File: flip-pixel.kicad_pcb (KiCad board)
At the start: 2 copper layers, 152.4 x 127 mm, 179 parts, among them J1 Barrel-Jack, Q1 DMN62D0U-7, Q10 STS8DN6LF6AG, Q11 DMN62D0U-7, Q12 DMN62D0U-7, Q13 STS8DN6LF6AG, Q14 DMN62D0U-7, Q15 DMN62D0U-7, Q16 STS8DN6LF6AG, Q17 DMN62D0U-7, Q18 DMN62D0U-7, Q19 STS8DN6LF6AG, Q2 DMN62D0U-7, Q20 DMN62D0U-7, Q21 DMN62D0U-7, Q22 STS8DN6LF6AG, Q23 DMN62D0U-7, Q24 DMN62D0U-7, Q25 STS8DN6LF6AG, Q26 DMN62D0U-7, Q27 DMN62D0U-7, Q28 STS8DN6LF6AG, Q29 DMN62D0U-7, Q3 DMN62D0U-7, Q30 DMN62D0U-7, Q31 STS8DN6LF6AG, Q4 STS8DN6LF6AG, Q5 DMN62D0U-7, Q6 DMN62D0U-7, Q7 STS8DN6LF6AG, Q8 DMN62D0U-7, Q9 DMN62D0U-7, U1 LM2665M6, U2 ESP32_DevBoard

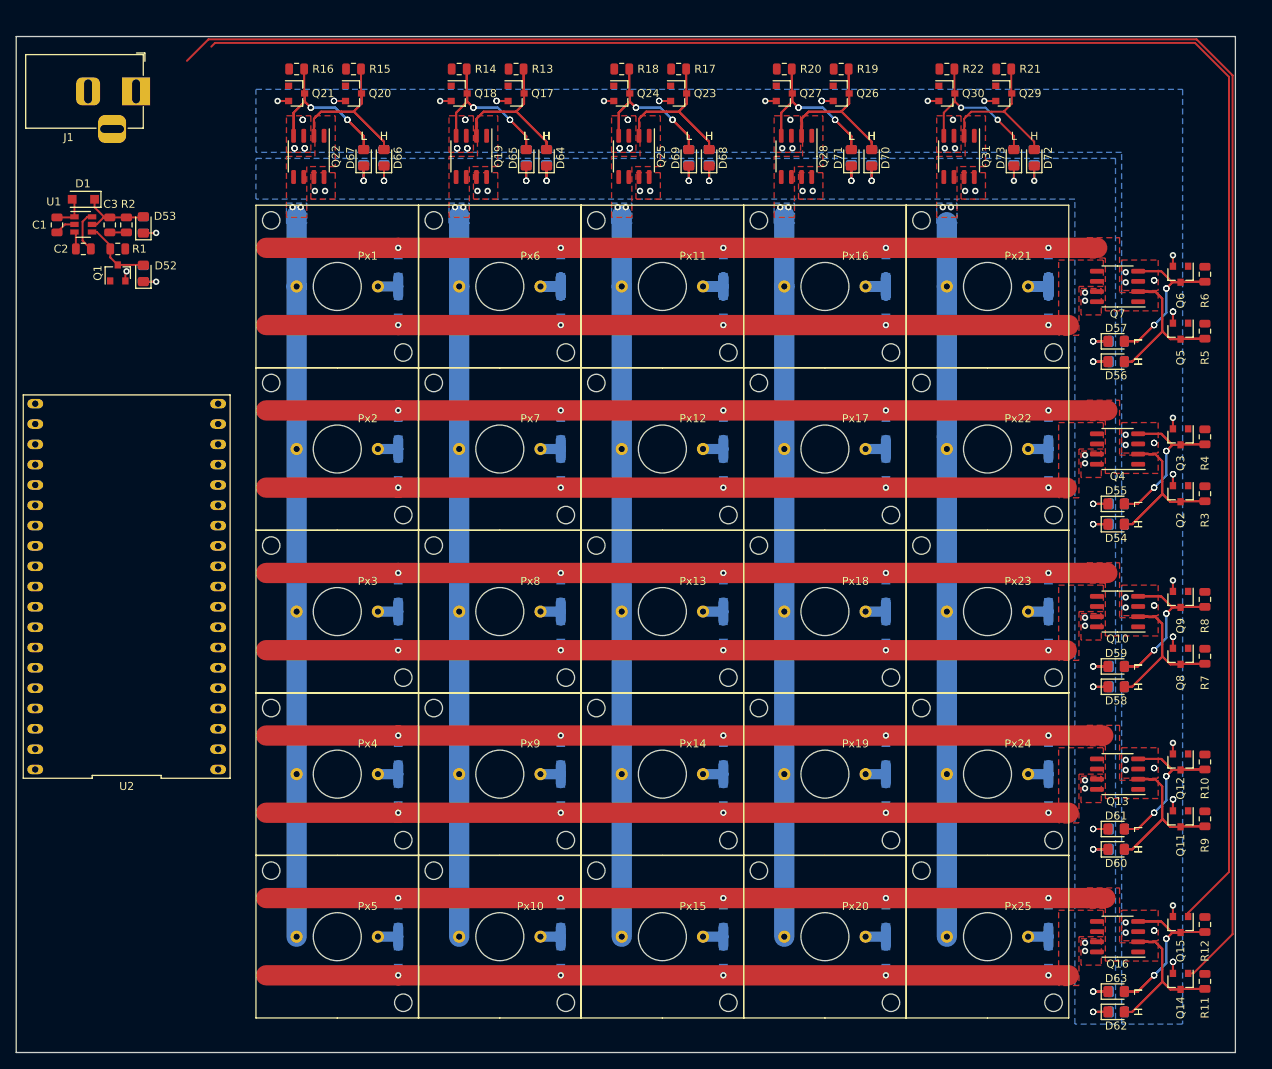
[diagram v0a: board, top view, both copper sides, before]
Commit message: starting trace routing
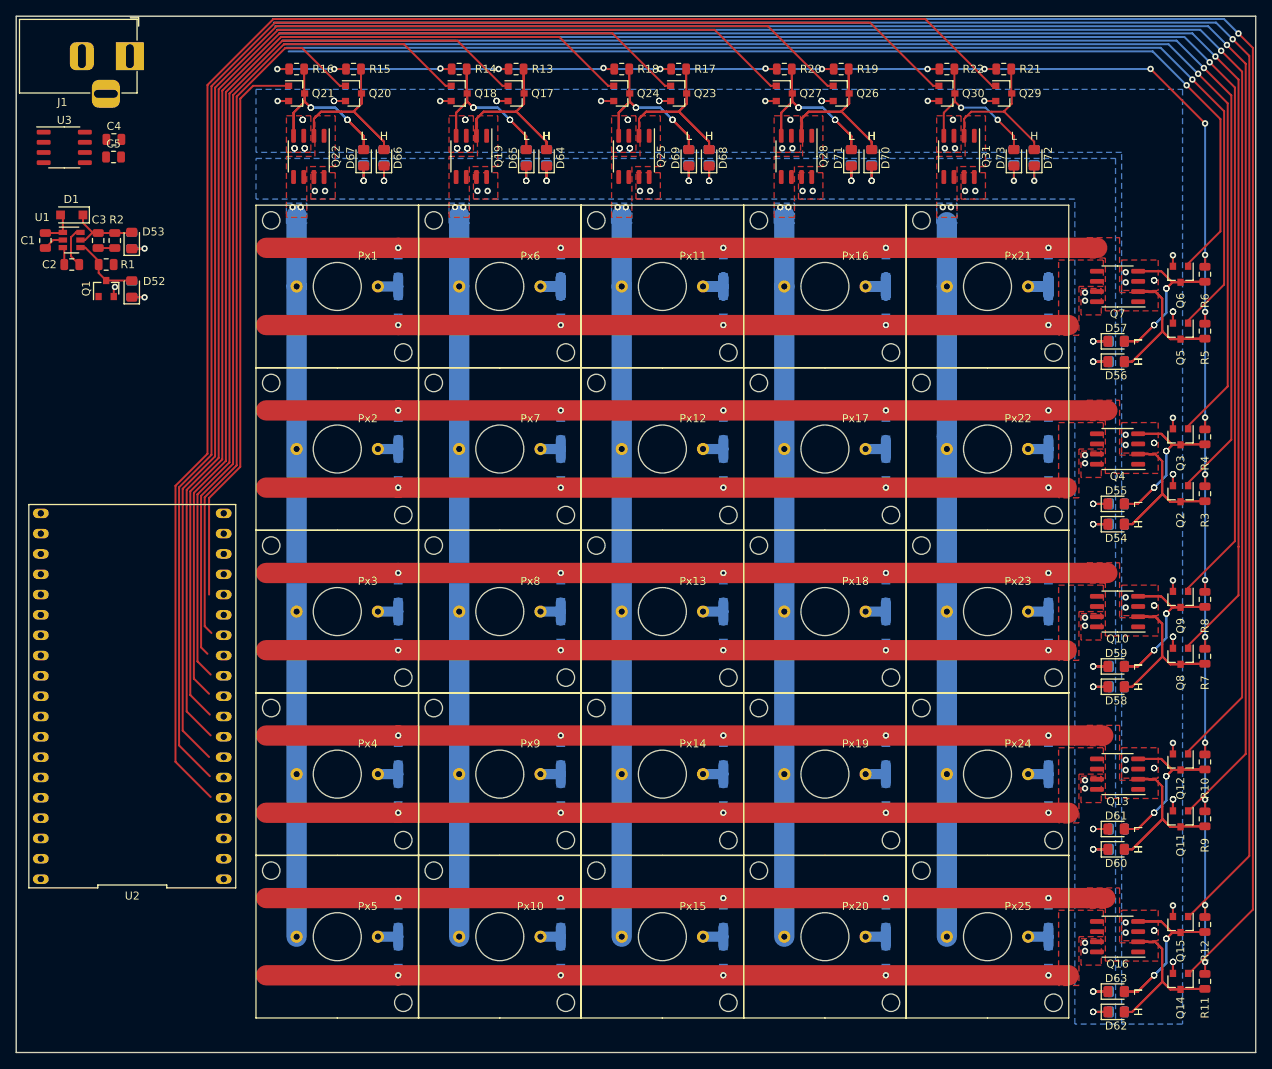
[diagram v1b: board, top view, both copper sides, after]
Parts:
- added C4: 0.1uF, Capacitor_SMD:C_0805_2012Metric, F.Cu at (110.0, 40.8)
- added C5: C, Capacitor_SMD:C_0805_2012Metric, F.Cu at (110.0, 43.0)
- added U3: ACS722, Custom-Footprints:SO-8_3.9x4.9mm_P1.27mm, F.Cu at (103.8, 41.8)
- moved U2 13.7 mm to (112.3, 110.4)
- moved J1 4.47 mm to (112.0, 30.4)
- moved D1 2.43 mm to (104.7, 50.2)
- moved C2 2.43 mm to (104.7, 56.4)
- moved C3 2.43 mm to (108.0, 53.4)
- moved D52 2.43 mm to (112.2, 59.5)
- moved D53 2.43 mm to (112.2, 53.4)
- moved Q1 2.43 mm to (109.0, 59.4)
- moved R1 2.43 mm to (109.0, 56.4)
- moved R2 2.43 mm to (110.1, 53.4)
- moved R23 2.43 mm to (112.2, 59.5)
- moved R24 2.43 mm to (112.2, 53.4)
- moved U1 2.43 mm to (104.7, 53.4)
- moved C1 2.43 mm to (101.4, 53.4)
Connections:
- J1 pad 1: +5V -> Net-(J1-Pad1)
- U2 pad 4: Net-(U2-Pad4) -> /current
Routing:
- net +10V: track 10.2 -> 262.9 mm, vias 0 -> 22
- net /Row4H: track 0.00 -> 219.7 mm, vias 0 -> 1
- net /Row4/Low_ct: track 0.00 -> 210.9 mm, vias 0 -> 1
- net /Col5H: track 0.00 -> 197.9 mm
- net /Row3H: track 0.00 -> 196.1 mm, vias 0 -> 1
- net /Row3/Low_ct: track 0.00 -> 187.3 mm, vias 0 -> 1
- net /Column5/Low_ct: track 0.00 -> 187.0 mm
- net /Row2H: track 0.00 -> 172.5 mm, vias 0 -> 1
- net /Col4H: track 0.00 -> 170.2 mm
- net /Row2/Low_ct: track 0.00 -> 163.8 mm, vias 0 -> 1
- net /Column4/Low_ct: track 0.00 -> 159.4 mm
- net /Row1H: track 0.00 -> 148.9 mm, vias 0 -> 1
- net /Col3H: track 0.00 -> 142.4 mm
- net /Row1/Low_ct: track 0.00 -> 140.1 mm, vias 0 -> 1
- net /Column3/Low_ct: track 0.00 -> 131.5 mm
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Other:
- board size 152.4 x 127 mm -> 154.9 x 129.5 mm
